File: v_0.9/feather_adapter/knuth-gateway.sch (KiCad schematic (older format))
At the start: 11 parts, among them J1 FeatherLora1, J2 FeatherLora2, J3 Conn_01x32_Male, J4 Conn_01x32_Male, J5 Conn_01x04_Female, J6 Conn_01x03_Female, J7 Conn_01x02_Female

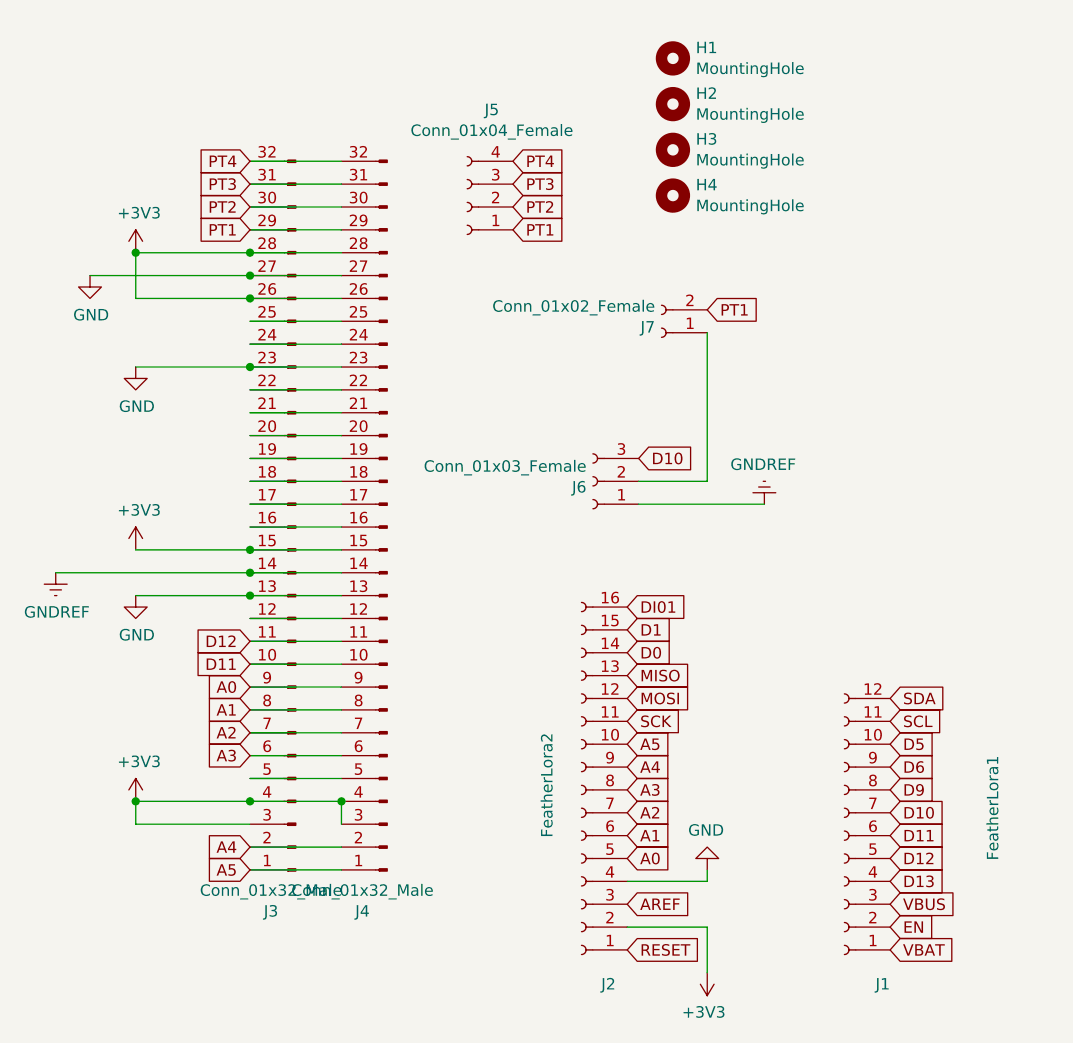
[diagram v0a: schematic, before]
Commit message: update ;
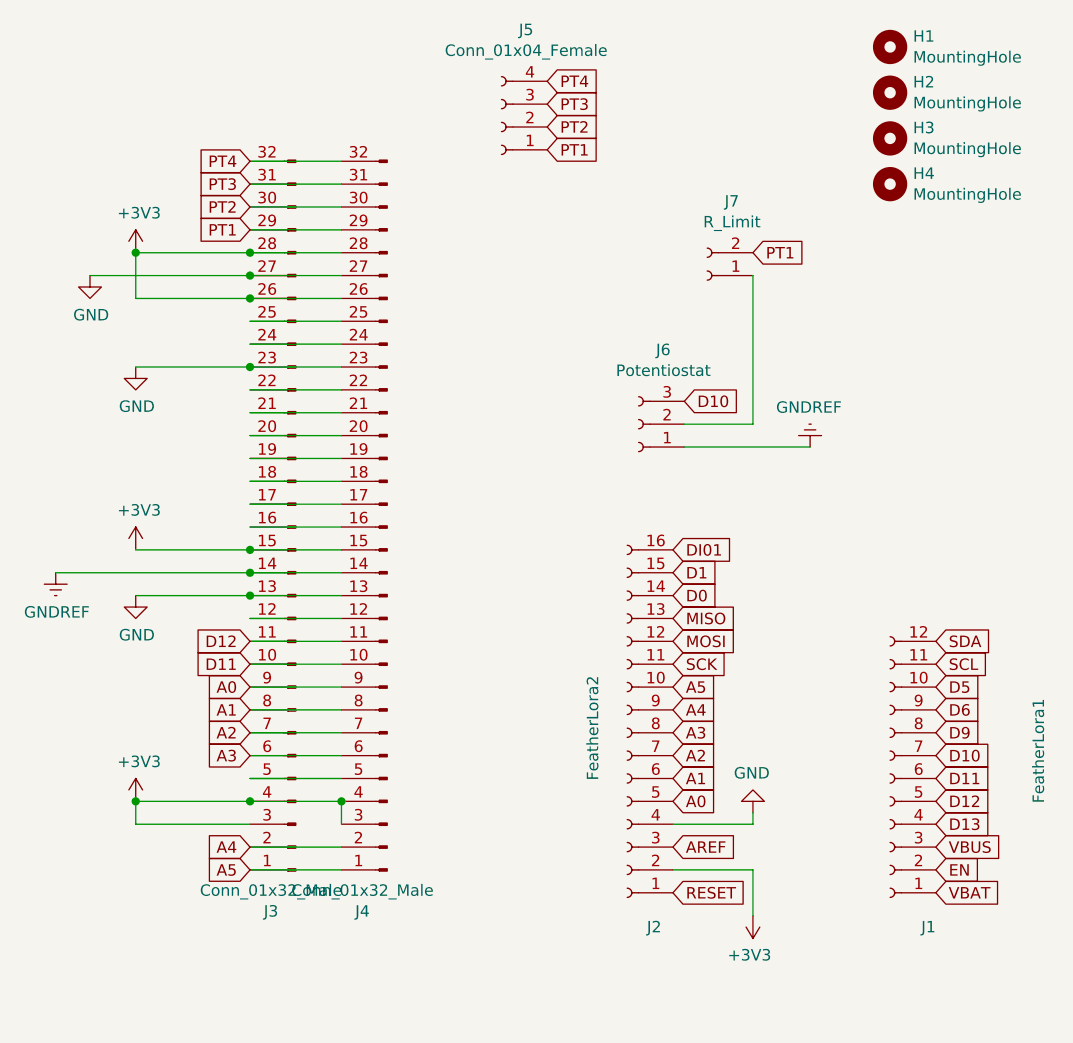
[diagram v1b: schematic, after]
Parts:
- J6: value Conn_01x03_Female -> Potentiostat
- J7: value Conn_01x02_Female -> R_Limit
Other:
- moved on the sheet: H1, H2, H3, H4, J1, J2, J5, J6, J7
